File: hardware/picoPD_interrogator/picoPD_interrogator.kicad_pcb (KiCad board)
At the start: 2 copper layers, 63.5 x 26 mm, 53 parts, among them J1 Conn_01x07, J2 USB_C_Receptacle_USB2.0_16P, J3 Conn_01x14, Q1 rohm-RE1C002UN, Q2 rohm-RE1C002UN, Q3 rohm-RE1C002UN, Q4 rohm-RE1C002UN, Q5 rohm-RE1C002UN, SW1 RESET_BTN, U3 ST-LM393QT, U6 LV2862XDDC

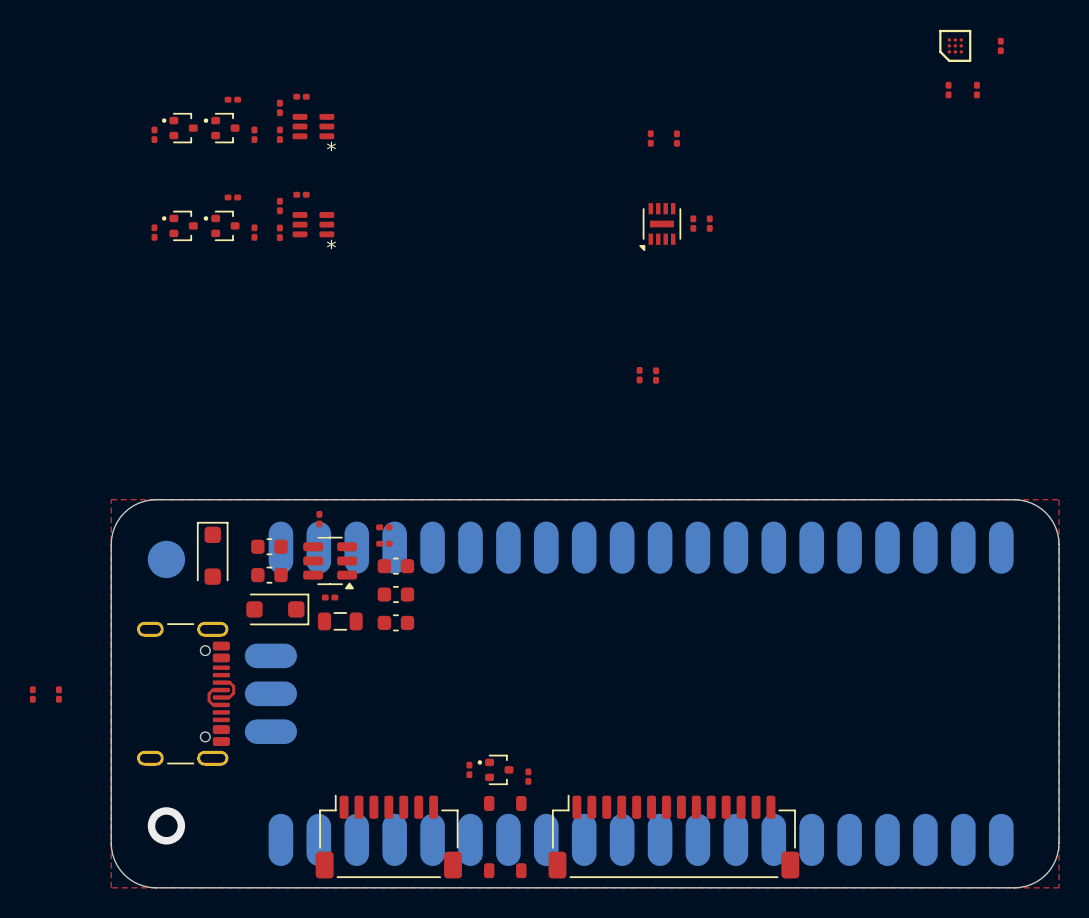
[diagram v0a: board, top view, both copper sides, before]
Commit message: PCB: Working on board layout.
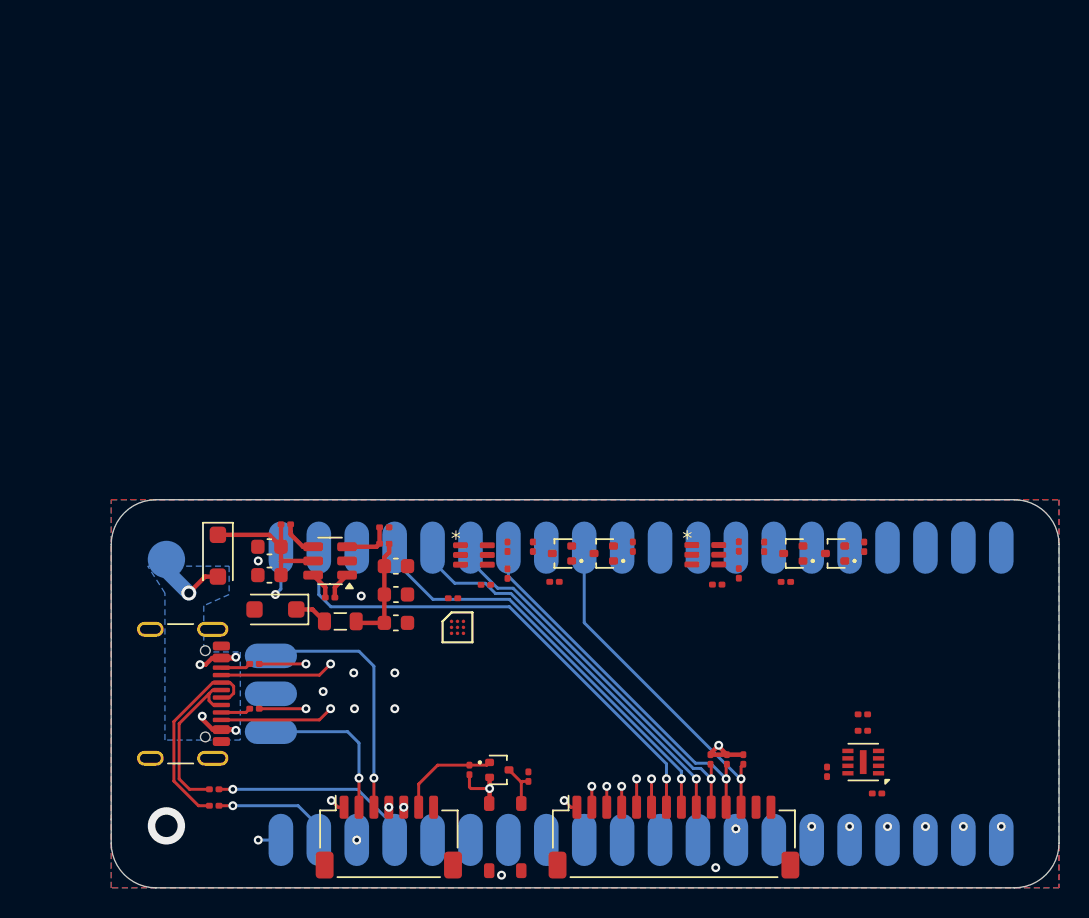
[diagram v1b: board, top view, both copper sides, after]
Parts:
- added R29: 3.3K, Resistor_SMD:R_0201_0603Metric, F.Cu at (156.8, 104.4)
- moved R7 52.1 mm to (137.4, 93.6), turned to 0 degrees
- moved R16 52.0 mm to (164.9, 90.2), turned to -90 degrees
- moved U1 51.3 mm to (137.7, 95.5), turned to 0 degrees
- moved Q5 48.9 mm to (163.0, 90.6), turned to 180 degrees
- moved R2 47.9 mm to (155.8, 104.4)
- moved R1 47.6 mm to (154.7, 104.4)
- moved R17 46.4 mm to (165.8, 106.7), turned to 0 degrees
- moved R19 45.1 mm to (159.7, 92.5), turned to 180 degrees
- moved Q4 43.9 mm to (160.2, 90.6), turned to 180 degrees
- moved R18 43.6 mm to (162.5, 105.2), turned to -90 degrees
- moved R11 42.3 mm to (149.4, 90.2), turned to -90 degrees
- moved R15 40.1 mm to (158.2, 90.2), turned to -90 degrees
- moved Q2 40.1 mm to (147.5, 90.6), turned to 180 degrees
- moved R3 39.4 mm to (156.6, 91.9), turned to 90 degrees
- moved R13 38.8 mm to (144.2, 92.5), turned to 180 degrees
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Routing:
- net /GP15: track 0.00 -> 41.4 mm, vias 0 -> 3
- net /GP16: track 0.00 -> 40.5 mm, vias 0 -> 3
- net /GP17: track 0.00 -> 33.1 mm, vias 0 -> 1
- net /GP18: track 0.00 -> 27.4 mm, vias 0 -> 1
- net /GP19: track 0.00 -> 25.6 mm, vias 0 -> 1
- net /SDA: track 0.00 -> 25.1 mm, vias 0 -> 1
- net /SCL: track 0.00 -> 24.1 mm, vias 0 -> 1
- net /SPI0_CLK: track 0.00 -> 23.1 mm, vias 0 -> 2
- net /TCPC_INT: track 0.00 -> 21.9 mm, vias 0 -> 1
- net /SPI0_MOSI: track 0.00 -> 19.2 mm, vias 0 -> 2
- net /SWD_CLK: track 0.00 -> 16.0 mm, vias 0 -> 1
- net /SPI0_MISO: track 0.00 -> 15.2 mm, vias 0 -> 2
- net /3V3: track 0.00 -> 13.3 mm, vias 0 -> 3
- net /PIO_USB_DP: track 0.00 -> 12.8 mm, vias 0 -> 1
- net /USB_DM_CONN: track 2.34 -> 13.7 mm
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- added copper zone on B.Cu, net /VBUS_CONN
- added copper zone on In2.Cu, net /VBUS_CONN
- added copper zone on B.Cu, net GND
- added copper zone on In1.Cu, net GND
- added copper zone on In2.Cu, net GND
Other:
- copper layers 2 -> 4
